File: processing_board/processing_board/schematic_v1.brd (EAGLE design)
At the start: 72.4 x 58.1 mm, 20 parts, among them Q1 BSS138, Q2 BSS138

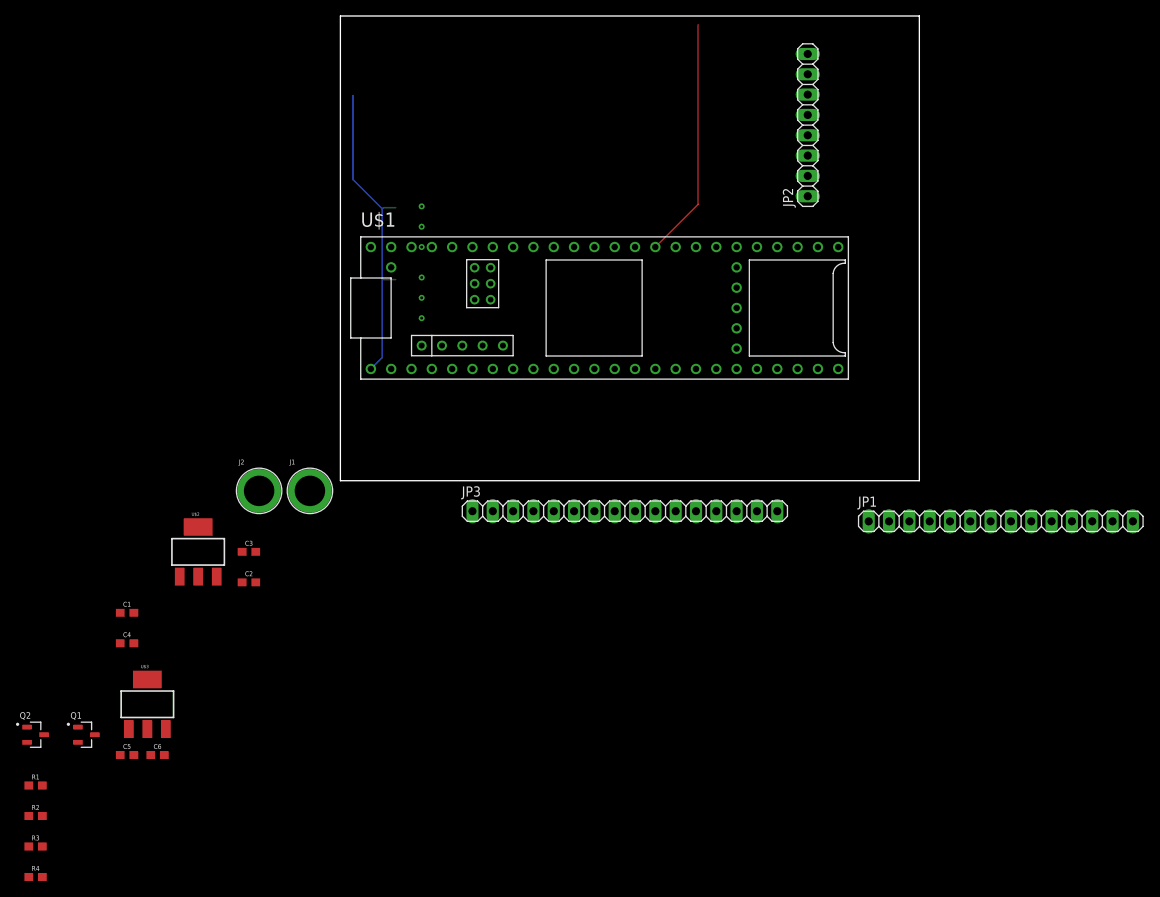
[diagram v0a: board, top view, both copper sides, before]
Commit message: modified shcematic and board
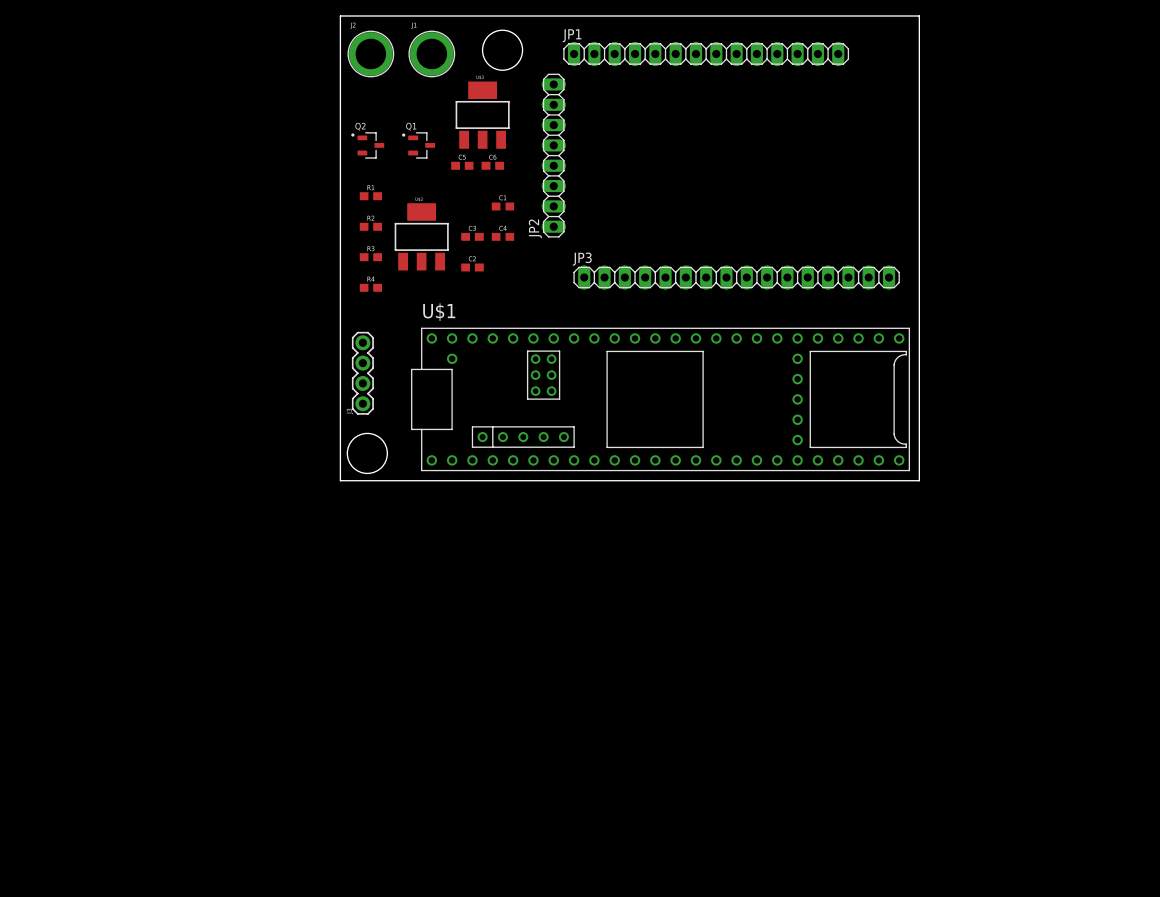
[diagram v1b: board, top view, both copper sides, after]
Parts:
- added J3: (no value), SparkFun-Connectors:1X04
- moved C5 84.7 mm to (14.0, 35.6)
- moved C6 84.7 mm to (17.8, 35.6)
- moved Q1 84.7 mm to (8.89, 38.1)
- moved Q2 84.7 mm to (2.54, 38.1)
- moved R1 84.7 mm to (2.54, 31.8)
- moved R2 84.7 mm to (2.54, 27.9)
- moved R3 84.7 mm to (2.54, 24.1)
- moved R4 84.7 mm to (2.54, 20.3)
- moved U$3 84.7 mm to (16.5, 41.9)
- moved C1 69.2 mm to (19.1, 30.5)
- moved C4 69.2 mm to (19.1, 26.7)
- moved JP1 69.1 mm to (44.5, 49.5)
- moved J1 56.7 mm to (10.2, 49.5)
- moved J2 56.4 mm to (2.54, 49.5)
- moved C2 48.3 mm to (15.2, 22.9)
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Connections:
- removed net N$11: Q2.2, R3.1
- removed net N$2: Q1.2, R2.1
- removed net VDD: C2.1, C3.2, U$1.VIN
- new net CAN_RX: J3.3, Q1.2, R2.1
- new net CAN_TX: J3.2, Q2.2, R3.1
- net +5V: now also C2.1, C3.2, J3.1, U$1.VIN
- net 3.3V: no longer U$1.3.3V
- net GND: now also J3.4
- net TEENSY_3.3V: now also U$1.3.3V
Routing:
- net GND: track 69.9 -> 0.50 mm
